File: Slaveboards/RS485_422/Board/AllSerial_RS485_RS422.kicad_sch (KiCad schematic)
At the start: 18 parts, among them IC1 7402D, IC2 MAX485CSA, IC3 MAX485CSA, IC4 MAX485CSA, IC5 MAX485CSA, J1 PinHeader_2x05_P2.54mm_Horizo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, X1 ALLSERIALSLAVE, X2 AKL18X-10W

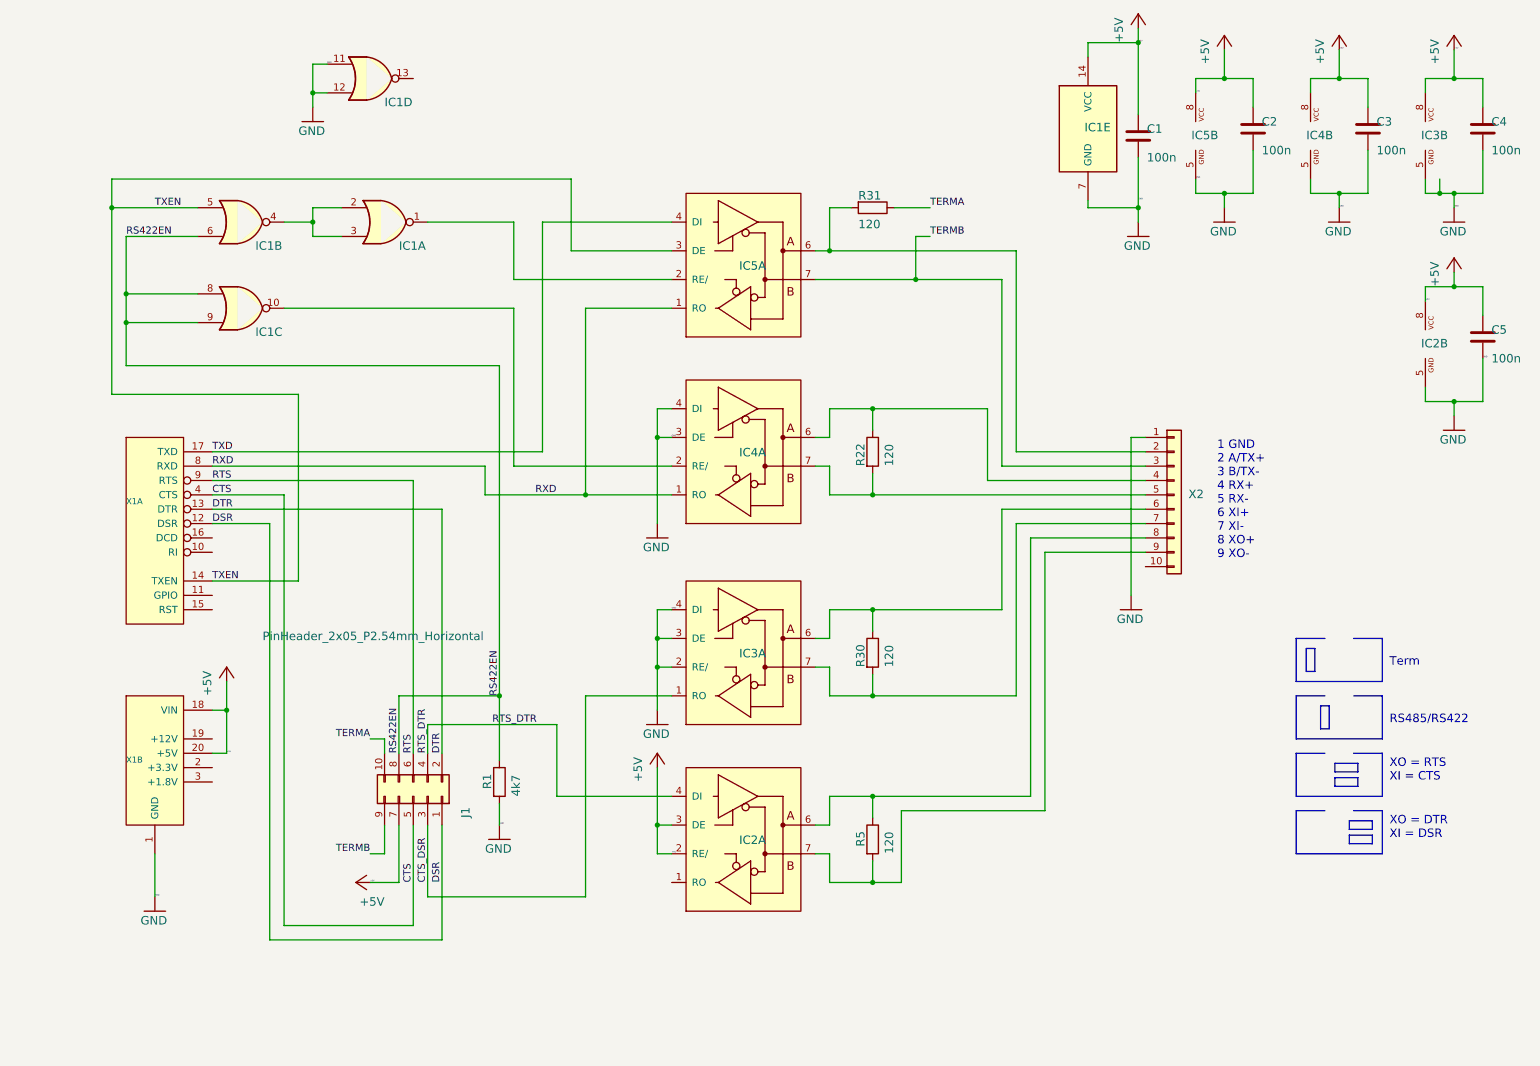
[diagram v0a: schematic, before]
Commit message: improve board/front links
clean up
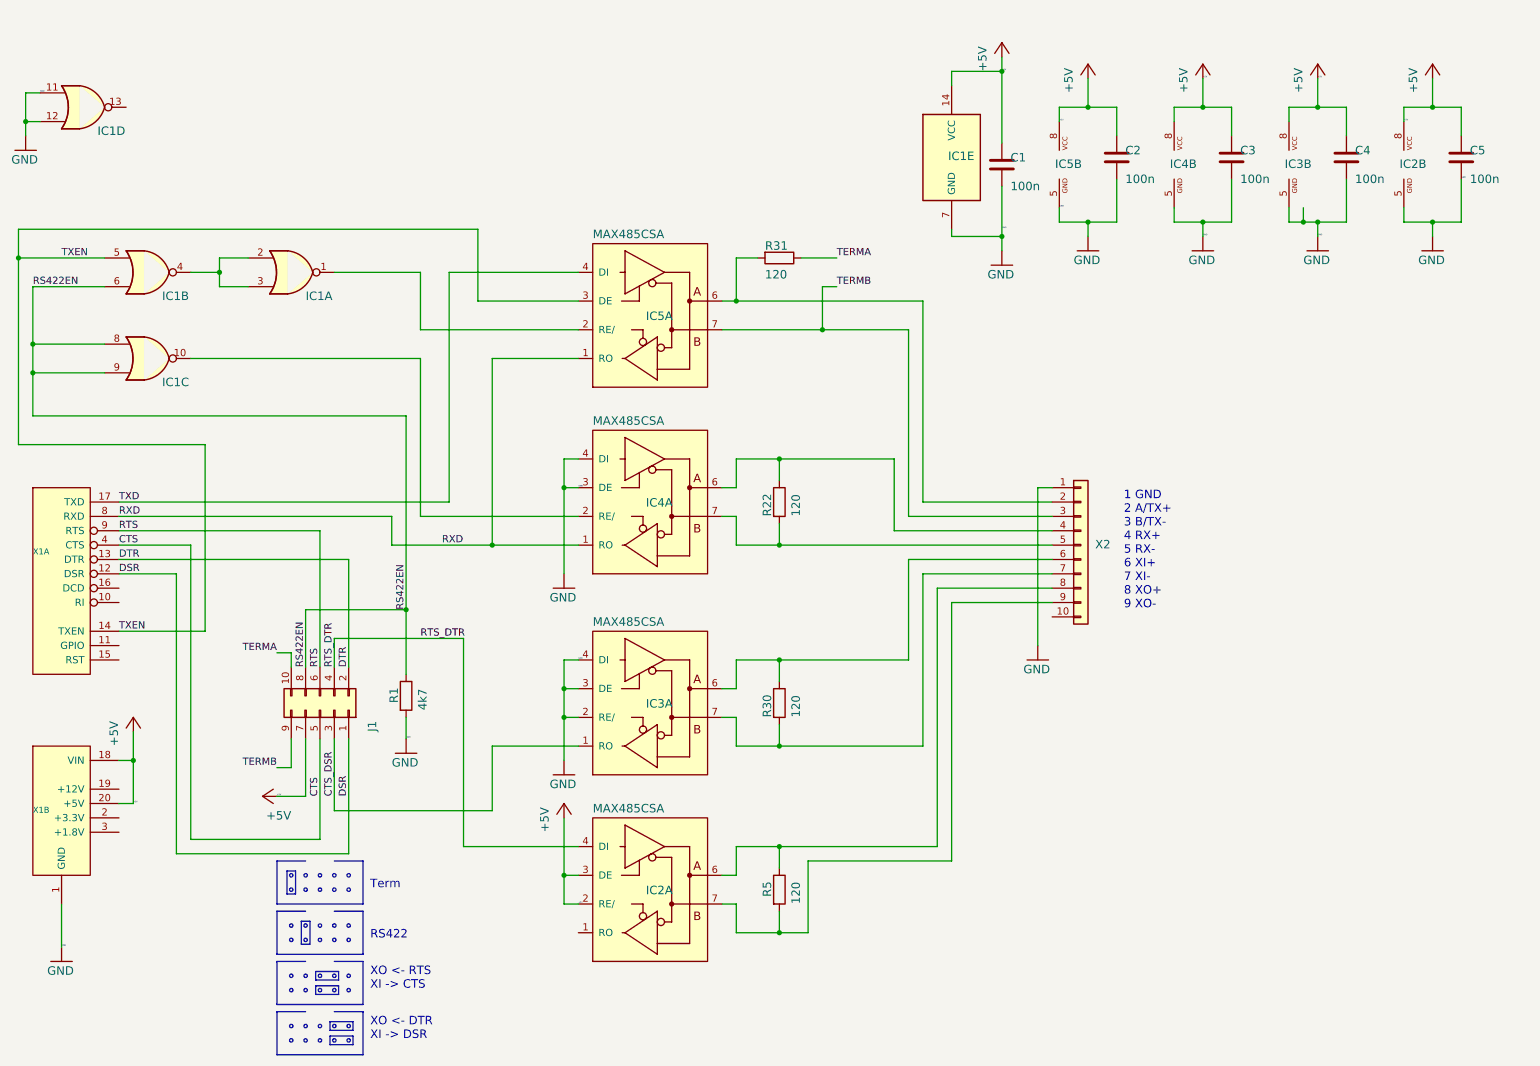
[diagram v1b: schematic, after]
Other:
- note added: "RS422"
- note added: "XO <- DTR XI -> DSR"
- note added: "XO <- RTS XI -> CTS"
- note removed: "RS485/RS422"
- note removed: "XO = DTR XI = DSR"
- note removed: "XO = RTS XI = CTS"
- moved on the sheet: C1, C2, C3, C4, C5, IC1A, IC1B, IC1C, IC1D, IC1E, IC2A, IC2B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
